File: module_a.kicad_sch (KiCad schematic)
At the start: 28 parts, among them J3 UART Activity Jumper, J5 Ethernet, J6 Micro_SD_Card_Det2, J7 nRPIBOOT Jumper, J8 RS232, U3 TPD4EUSB30, U4 TPD4EUSB30, U5 MAX3232, U6 RT9742GGJ5

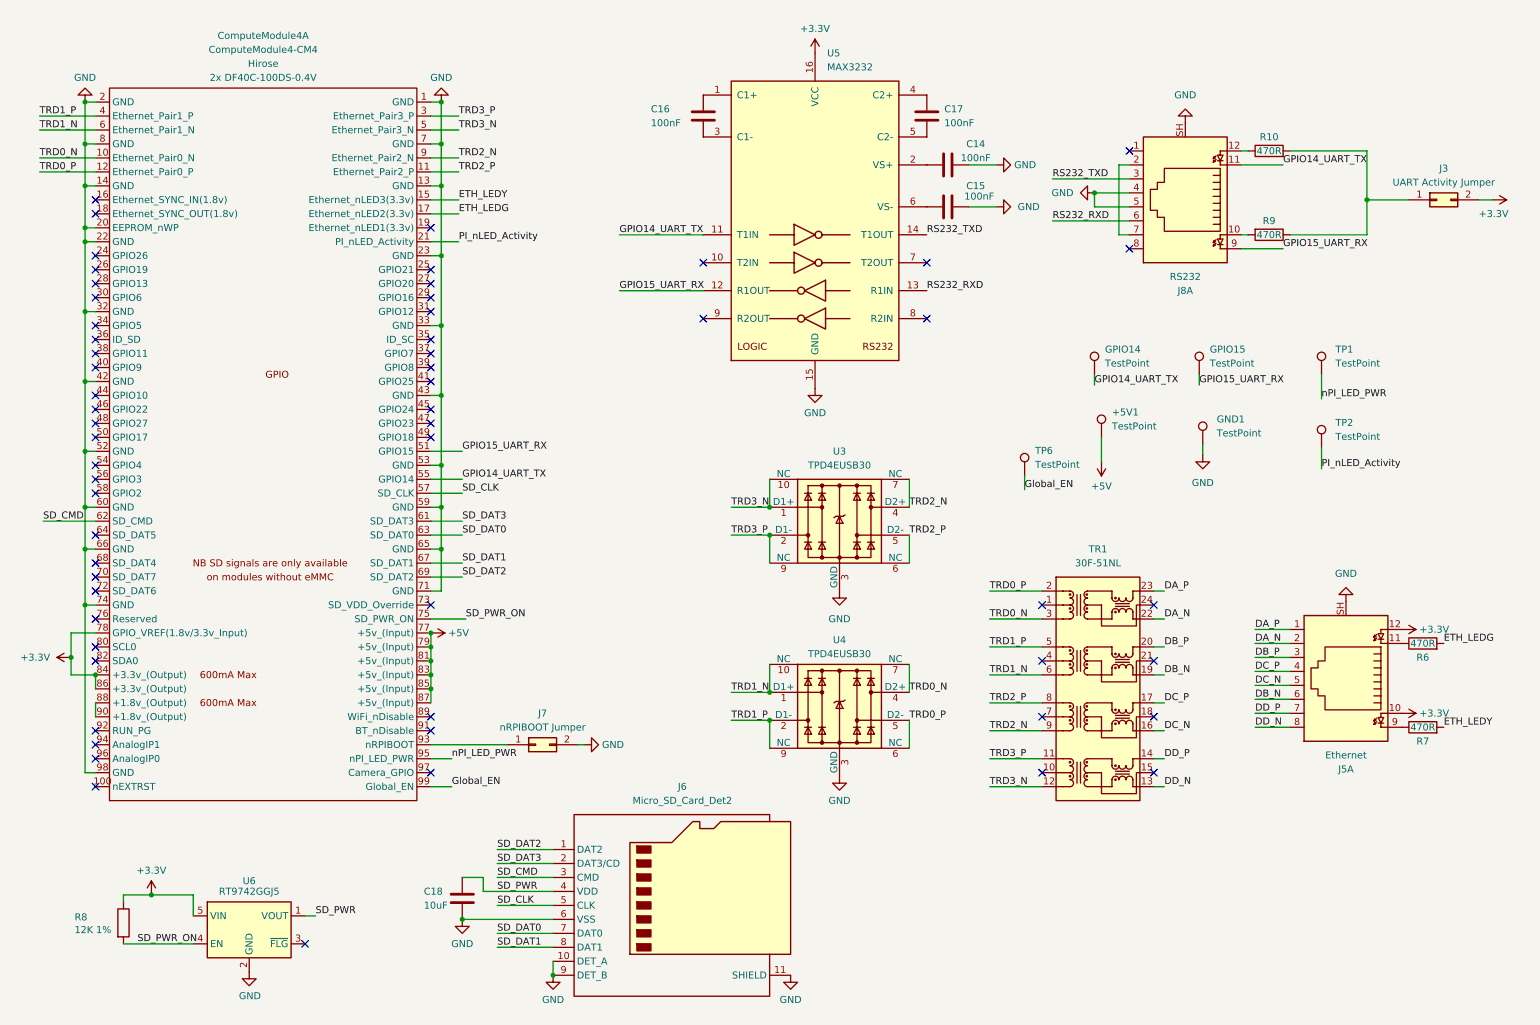
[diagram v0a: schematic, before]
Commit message: PiCard v2
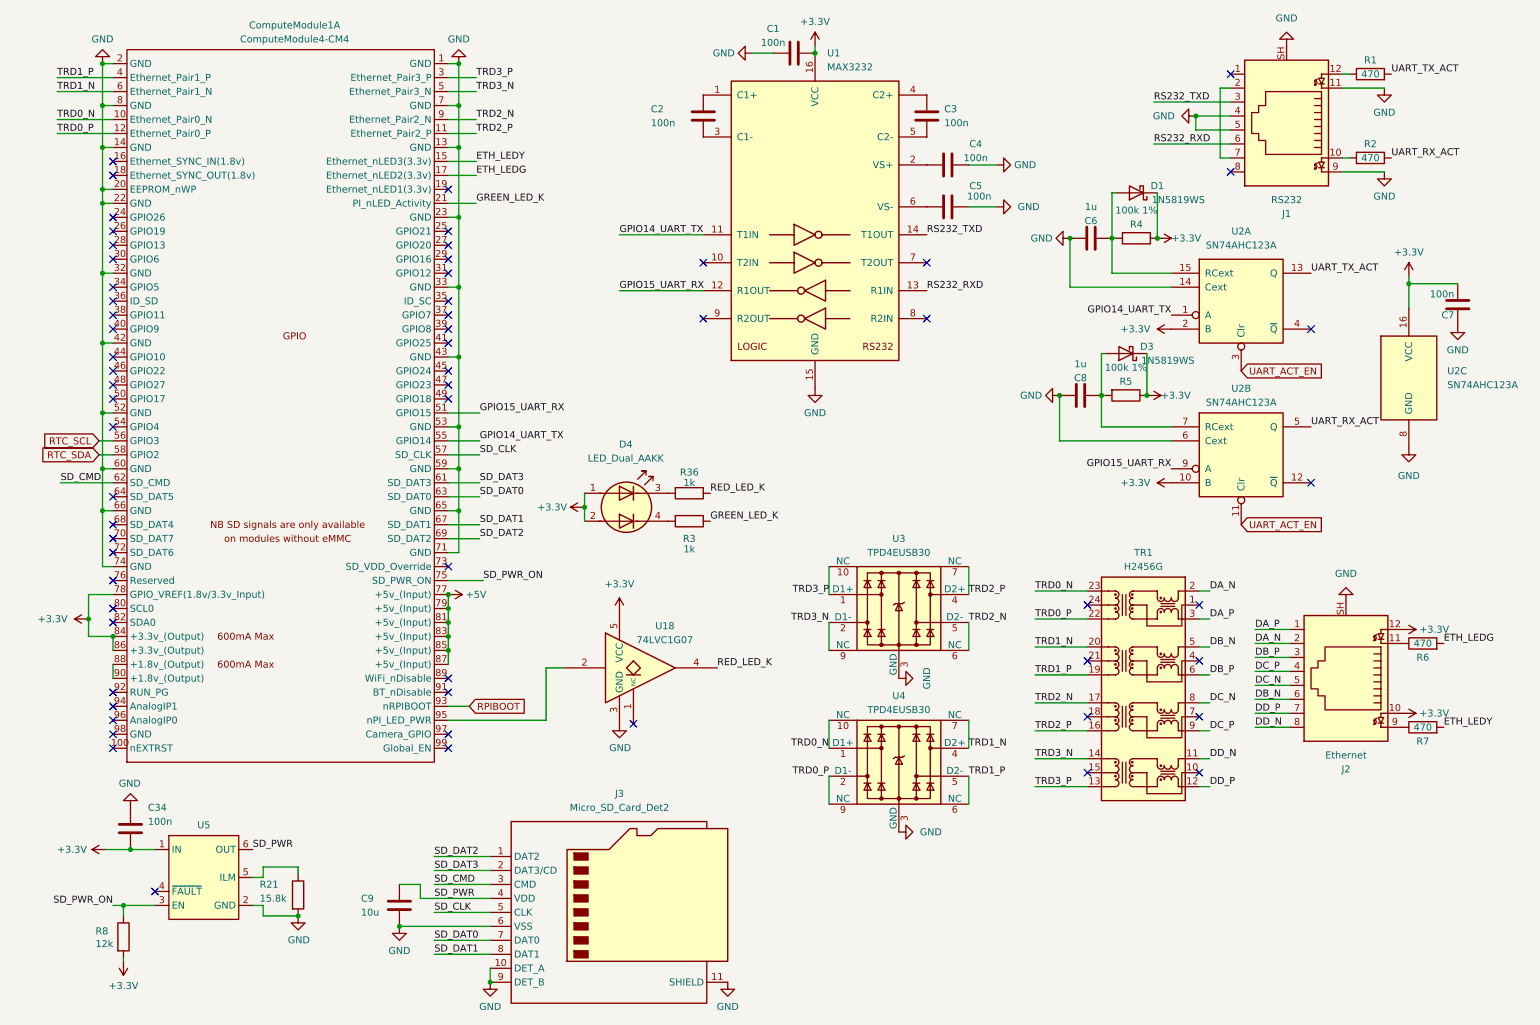
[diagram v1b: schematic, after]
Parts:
- removed +5V1, GND1, GPIO14, GPIO15, TP1, TP2, TP6: TestPoint, TestPoint:TestPoint_Pad_D2.0mm, symbol Connector:TestPoint
- removed J3: UART Activity Jumper, Connector_PinHeader_2.00mm:PinHeader_1x02_P2.00mm_Vertical, symbol Connector_Generic:Conn_02x01
- removed J7: nRPIBOOT Jumper, Connector_PinHeader_2.00mm:PinHeader_1x02_P2.00mm_Vertical, symbol Connector_Generic:Conn_02x01
- removed TR1: 30F-51NL, Transformer_SMD:Transformer_Ethernet_YDS_30F-51NL_SO-24_7.1x15.1mm, symbol Transformer:30F-51NL
- removed U6: RT9742GGJ5, Package_TO_SOT_SMD:TSOT-23-5, symbol PiCard:RT9742GGJ5F
- added C1, C34, C7: 100n, Capacitor_SMD:C_0402_1005Metric, symbol Device:C
- added C6, C8: 1u, Capacitor_SMD:C_0603_1608Metric, symbol Device:C
- added D1, D3: 1N5819WS, Diode_SMD:D_SOD-323, symbol Device:D_Schottky
- added D4: LED_Dual_AAKK, PiCard:LED-ARRAY-SMD_4P-L3.0-W1.5-L-FD, symbol Device:LED_Dual_AAKK
- added R21: 15.8k, Resistor_SMD:R_0402_1005Metric, symbol Device:R
- added R3, R36: 1k, Resistor_SMD:R_0402_1005Metric, symbol Device:R
- added R4, R5: 100k 1%, Resistor_SMD:R_0402_1005Metric, symbol Device:R
- added TR1: H2456G, PiCard:XFMR-SMD-24_L16.6-W9.0-LS9.6-BL, symbol Magi:H2456G
- added U18: 74LVC1G07, Package_TO_SOT_SMD:SOT-353_SC-70-5, symbol 74xGxx:74LVC1G07
- added U2: SN74AHC123A, Package_SO:TSSOP-16_4.4x5mm_P0.65mm, symbol 74xx:74AHCT123
- added U5: ~, Package_TO_SOT_SMD:SOT-23-6, symbol PiCard:TPS2553
- C2: renamed from C16; value 100nF -> 100n; footprint Capacitor_SMD:C_0603_1608Metric -> Capacitor_SMD:C_0402_1005Metric; LCSC C45000 -> C307331; MPN (none) -> CL05B104KB54PNC; Manufacturer (none) -> Samsung
- C3: renamed from C17; value 100nF -> 100n; footprint Capacitor_SMD:C_0603_1608Metric -> Capacitor_SMD:C_0402_1005Metric; LCSC C45000 -> C307331; MPN (none) -> CL05B104KB54PNC; Manufacturer (none) -> Samsung
- C4: renamed from C14; value 100nF -> 100n; footprint Capacitor_SMD:C_0603_1608Metric -> Capacitor_SMD:C_0402_1005Metric; LCSC C45000 -> C307331; MPN (none) -> CL05B104KB54PNC; Manufacturer (none) -> Samsung
- C5: renamed from C15; value 100nF -> 100n; footprint Capacitor_SMD:C_0603_1608Metric -> Capacitor_SMD:C_0402_1005Metric; LCSC C45000 -> C307331; MPN (none) -> CL05B104KB54PNC; Manufacturer (none) -> Samsung
- C9: renamed from C18; value 10uF -> 10u; LCSC C2167686 -> C15850; MPN (none) -> CL21A106KAYNNNE; Manufacturer (none) -> C15850
- J1: renamed from J8; footprint PiCard:RJ45-TH_MJ88B-B011-RVL11-P -> PiCard:RJ45-TH_RJ45-005-202-11; symbol Connector:RJ45_LED_Shielded_x2 -> Connector:RJ45_LED_Shielded; LCSC C501462 -> C7421405; MPN (none) -> RJ45-005-202-11; Manufacturer (none) -> Heling
- J2: renamed from J5; footprint PiCard:RJ45-TH_MJ88B-B011-RVL11-P -> PiCard:RJ45-TH_RJ45-005-202-11; symbol Connector:RJ45_LED_Shielded_x2 -> Connector:RJ45_LED_Shielded; LCSC C501462 -> C7421405; MPN (none) -> RJ45-005-202-11; Manufacturer (none) -> Heling
- J3: renamed from J6; LCSC (none) -> C5174683; LCSC Part # C5174683 -> (none); MPN (none) -> TF-108-ARP10; Manufacturer (none) -> XUNPU
- R1: renamed from R10; value 470R -> 470; footprint Resistor_SMD:R_0805_2012Metric -> Resistor_SMD:R_0402_1005Metric; LCSC C17710 -> C25117; MPN (none) -> 0402WGF4700TCE; Manufacturer (none) -> Uniroyal
- R2: renamed from R9; value 470R -> 470; footprint Resistor_SMD:R_0805_2012Metric -> Resistor_SMD:R_0402_1005Metric; LCSC C17710 -> C25117; MPN (none) -> 0402WGF4700TCE; Manufacturer (none) -> Uniroyal
- R6, R7: value 470R -> 470; footprint Resistor_SMD:R_0805_2012Metric -> Resistor_SMD:R_0402_1005Metric; LCSC C17710 -> C25117; MPN (none) -> 0402WGF4700TCE; Manufacturer (none) -> Uniroyal
- R8: value 12K 1% -> 12k; footprint Resistor_SMD:R_0805_2012Metric -> Resistor_SMD:R_0402_1005Metric; LCSC C17444 -> C25752; MPN (none) -> 0402WGF1202TCE; Manufacturer (none) -> Uniroyal
- U1: renamed from U5; footprint PiCard:TSSOP-16_L5.0-W4.4-P0.65-LS6.4-BL -> Package_SO:TSSOP-16_4.4x5mm_P0.65mm; MPN (none) -> MAX3232EEUE+T; Manufacturer (none) -> Maxim
- U3, U4: MPN (none) -> TPD4EUSB30DQAR; Manufacturer (none) -> Texas Instruments
- renumbered ComputeModule4 to ComputeModule1
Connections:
- net +3.3V: now also R8.2, C1.2, C34.2, C7.2, D1.1 (K), D3.1 (K), D4.1 (A1), D4.2 (A2), R4.1, R5.1, U18.5 (VCC), U2.10 (B), U2.16 (VCC), U2.2 (B), U5.1 (IN); no longer R8.1
- net DA_N: now also TR1.2 (MX1+)
- net DA_P: now also TR1.3 (MX1-)
- net DB_N: now also TR1.5 (MX2+)
- net DB_P: now also TR1.6 (MX2-)
- net DC_N: now also TR1.8 (MX3+)
- net DC_P: now also TR1.9 (MX3-)
- net DD_N: now also TR1.11 (MX4+)
- net DD_P: now also TR1.12 (MX4-)
- net GND: now also J1.11, J1.9, C1.1, C34.1, C6.2, C7.1, C8.2, R21.2, U18.3 (GND), U2.14 (Cext), U2.6 (Cext), U2.8 (GND), U5.2 (GND); no longer ComputeModule1.98 (GND)
- net GPIO14_UART_TX: now also U2.1 (A); no longer J1.11
- net GPIO15_UART_RX: now also U2.9 (A); no longer J1.9
- net SD_PWR: now also U5.6 (OUT)
- net SD_PWR_ON: now also R8.1, U5.3 (EN); no longer R8.2
- net TRD0_N: now also U4.1 (D1+), U4.10 (NC), TR1.23 (TD1+); no longer U4.4 (D2+), U4.7 (NC)
- net TRD0_P: now also U4.2 (D1-), U4.9 (NC), TR1.22 (TD1-); no longer U4.5 (D2-), U4.6 (NC)
- net TRD1_N: now also U4.4 (D2+), U4.7 (NC), TR1.20 (TD2+); no longer U4.1 (D1+), U4.10 (NC)
- net TRD1_P: now also U4.5 (D2-), U4.6 (NC), TR1.19 (TD2-); no longer U4.2 (D1-), U4.9 (NC)
- net TRD2_N: now also U3.5 (D2-), U3.6 (NC), TR1.17; no longer U3.4 (D2+), U3.7 (NC)
- net TRD2_P: now also U3.4 (D2+), U3.7 (NC), TR1.16 (TD3-); no longer U3.5 (D2-), U3.6 (NC)
- net TRD3_N: now also U3.2 (D1-), U3.9 (NC), TR1.14 (TD4+); no longer U3.1 (D1+), U3.10 (NC)
- net TRD3_P: now also U3.1 (D1+), U3.10 (NC), TR1.13 (TD4-); no longer U3.2 (D1-), U3.9 (NC)
- net RTC_SCL: now reaches ComputeModule1.56 (GPIO3)
- net RTC_SDA: now reaches ComputeModule1.58 (GPIO2)
- net RPIBOOT: now reaches ComputeModule1.93 (nRPIBOOT)
- net UART_RX_ACT: now reaches R2.1
- net UART_RX_ACT: now also U2.5 (Q); no longer R1.2
- net Global_EN: no longer names the net of ComputeModule1.99 (Global_EN)
- net PI_nLED_Activity renamed GREEN_LED_K
- net GREEN_LED_K: now also R3.1
- net nPI_LED_PWR: no longer names the net of ComputeModule1.95 (nPI_LED_PWR)
- net nPI_LED_PWR: now also U18.2
- new net: R21.1, U5.5 (ILM)
- new net: C6.1, D1.2 (A), R4.2, U2.15 (RCext)
- new net: C8.1, D3.2 (A), R5.2, U2.7 (RCext)
- new net: D4.3 (K1), R36.2
- new net: D4.4 (K2), R3.2
- new net RED_LED_K: R36.1, U18.4
- new net UART_ACT_EN: U2.11 (Clr), U2.3 (Clr)
- new net UART_TX_ACT: R1.2, U2.13 (Q)
- no-connect marks 59 -> 62
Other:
- moved on the sheet: C9, ComputeModule1A, J1, J3, R1, R2, U3, U4
